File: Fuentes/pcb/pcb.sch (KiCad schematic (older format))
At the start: 16 parts, among them P1 entrada1, P2 entrada 2, P3 +50V, P4 -50V

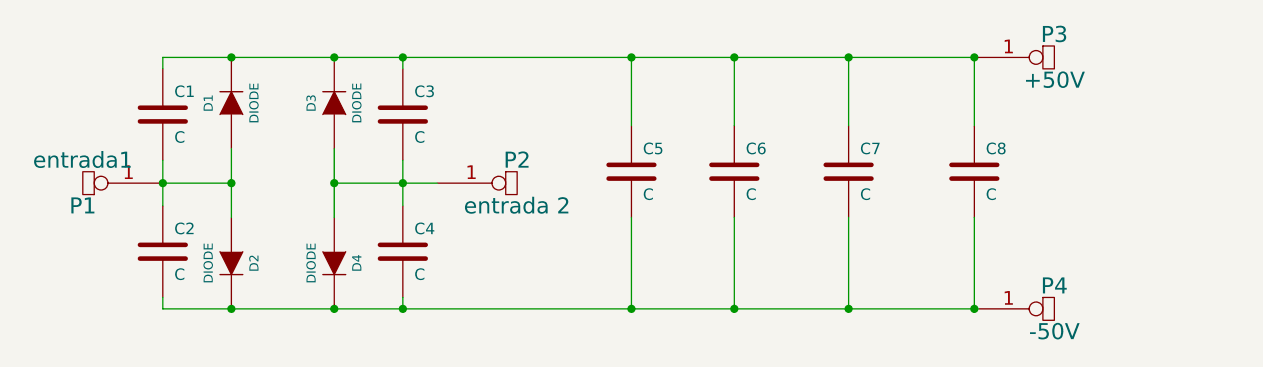
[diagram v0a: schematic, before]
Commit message: subo pcb de la fuente lineal 3
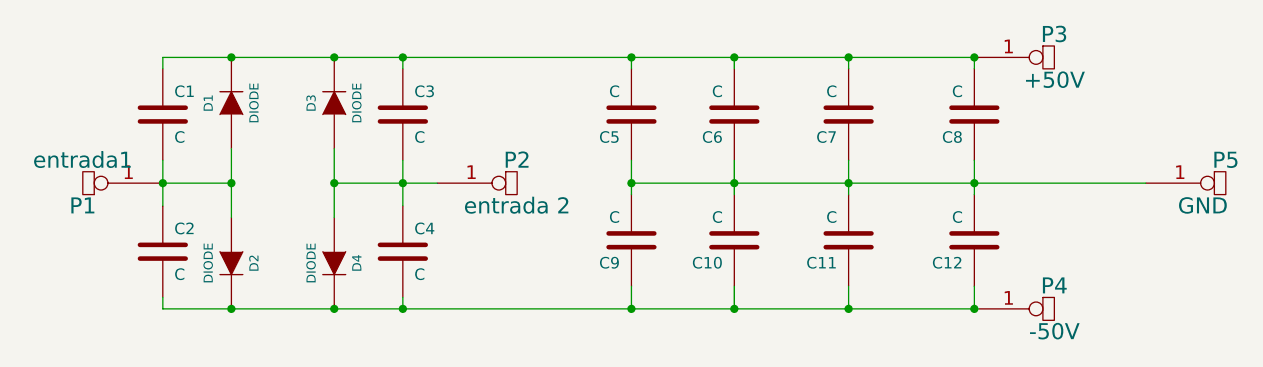
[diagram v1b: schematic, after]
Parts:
- added C10, C11, C12, C9: C, symbol C
- added P5: GND, symbol CONNECTOR
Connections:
- net at C1.1, C3.1, D1.2 (K)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: now also C5.2, C6.2, C7.2, C8.2; no longer C5.1, C6.1, C7.1, C8.1
- net at C2.2, C4.2, D2.2 (K)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: now also C10.1, C11.1, C12.1, C9.1; no longer C5.2, C6.2, C7.2, C8.2
- new net: C10.2, C11.2, C12.2, C5.1, C6.1, C7.1, C8.1, C9.2, P5.1 (W)
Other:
- moved on the sheet: C5, C6, C7, C8
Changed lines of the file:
@@
-EESchema Schematic File Version 2  date jue 31 may 2012 13:24:02 ART
+EESchema Schematic File Version 2  date jue 31 may 2012 14:37:13 ART
 LIBS:power
 LIBS:device
@@
 Comment4 ""
 $EndDescr
+Wire Wire Line
+	3200 1200 3200 1250
+Wire Wire Line
+	4700 1250 4700 1200
+Wire Wire Line
+	3200 2200 3200 2300
+Wire Wire Line
+	4150 2300 4150 2200
+Wire Wire Line
+	3650 1650 3650 1800
+Wire Wire Line
+	4700 1800 4700 1650
+Wire Wire Line
+	3200 1800 3200 1650
+Connection ~ 4150 1200
+Connection ~ 3650 2300
+Connection ~ 3200 1200
+Wire Wire Line
+	4700 1200 1150 1200
+Connection ~ 2200 2300
+Wire Wire Line
+	2200 2300 2200 2250
+Connection ~ 1450 2300
+Wire Wire Line
+	1150 2250 1150 2300
+Wire Wire Line
+	2200 1650 2200 1850
+Wire Wire Line
+	1150 1650 1150 1850
+Connection ~ 1900 1750
+Wire Wire Line
+	1900 1750 2350 1750
+Wire Wire Line
+	1450 1600 1450 1900
+Wire Wire Line
+	1900 1900 1900 1600
+Wire Wire Line
+	1450 1750 1150 1750
+Connection ~ 1450 1750
+Wire Wire Line
+	1150 1200 1150 1250
+Connection ~ 1450 1200
+Wire Wire Line
+	2200 1250 2200 1200
+Connection ~ 2200 1200
+Connection ~ 2200 1750
+Connection ~ 1150 1750
+Connection ~ 1900 2300
+Connection ~ 1900 1200
+Connection ~ 3200 2300
+Wire Wire Line
+	1150 2300 4700 2300
+Connection ~ 4150 2300
+Connection ~ 3650 1200
+Connection ~ 4700 2300
 Connection ~ 4700 1200
-Connection ~ 4700 2300
+Wire Wire Line
+	3200 1750 5450 1750
+Connection ~ 3200 1750
+Wire Wire Line
+	4150 1800 4150 1650
+Wire Wire Line
+	3650 2200 3650 2300
+Wire Wire Line
+	4700 2300 4700 2200
+Connection ~ 4700 1750
+Connection ~ 4150 1750
+Connection ~ 3650 1750
+Wire Wire Line
+	4150 1250 4150 1200
+Wire Wire Line
+	3650 1250 3650 1200
+$Comp
+L CONNECTOR P5
+U 1 1 4FC7AB52
+P 5450 1750
+F 0 "P5" H 5800 1850 70  0000 C CNN
+F 1 "GND" H 5700 1650 70  0000 C CNN
+	1    5450 1750
+	1    0    0    -1
+$EndComp
+$Comp
+L C C9
+U 1 1 4FC7AB35
+P 3200 2000
+F 0 "C9" H 3250 2100 50  0000 L CNN
+F 1 "C" H 3250 1900 50  0000 L CNN
+	1    3200 2000
+	-1   0    0    1
+$EndComp
+$Comp
+L C C10
+U 1 1 4FC7AB34
+P 3650 2000
+F 0 "C10" H 3700 2100 50  0000 L CNN
+F 1 "C" H 3700 1900 50  0000 L CNN
+	1    3650 2000
+	-1   0    0    1
+$EndComp
+$Comp
+L C C11
+U 1 1 4FC7AB33
+P 4150 2000
+F 0 "C11" H 4200 2100 50  0000 L CNN
+F 1 "C" H 4200 1900 50  0000 L CNN
+	1    4150 2000
+	-1   0    0    1
+$EndComp
+$Comp
+L C C12
+U 1 1 4FC7AB32
+P 4700 2000
+F 0 "C12" H 4750 2100 50  0000 L CNN
+F 1 "C" H 4750 1900 50  0000 L CNN
+	1    4700 2000
+	-1   0    0    1
+$EndComp
 $Comp
 L CONNECTOR P3
@@
 	1    0    0    -1
 $EndComp
-Connection ~ 3650 1200
-Wire Wire Line
-	3650 1500 3650 1200
-Connection ~ 4150 2300
-Wire Wire Line
-	4700 2300 1150 2300
-Wire Wire Line
-	4700 2300 4700 1900
-Connection ~ 3200 2300
-Wire Wire Line
-	3650 2300 3650 1900
-Connection ~ 1900 1200
-Wire Wire Line
-	3200 1200 3200 1500
-Connection ~ 1900 2300
-Connection ~ 1150 1750
-Connection ~ 2200 1750
-Connection ~ 2200 1200
-Wire Wire Line
-	2200 1250 2200 1200
-Connection ~ 1450 1200
-Wire Wire Line
-	1150 1250 1150 1200
-Connection ~ 1450 1750
-Wire Wire Line
-	1450 1750 1150 1750
-Wire Wire Line
-	1900 1900 1900 1600
-Wire Wire Line
-	1450 1600 1450 1900
-Wire Wire Line
-	1900 1750 2350 1750
-Connection ~ 1900 1750
-Wire Wire Line
-	1150 1650 1150 1850
-Wire Wire Line
-	2200 1650 2200 1850
-Wire Wire Line
-	1150 2300 1150 2250
-Connection ~ 1450 2300
-Wire Wire Line
-	2200 2300 2200 2250
-Connection ~ 2200 2300
-Wire Wire Line
-	3200 2300 3200 1900
-Wire Wire Line
-	4700 1500 4700 1200
-Wire Wire Line
-	4700 1200 1150 1200
-Connection ~ 3200 1200
-Wire Wire Line
-	4150 2300 4150 1900
-Connection ~ 3650 2300
-Wire Wire Line
-	4150 1500 4150 1200
-Connection ~ 4150 1200
 $Comp
 L C C8
 U 1 1 4FC785F8
-P 4700 1700
-F 0 "C8" H 4750 1800 50  0000 L CNN
-F 1 "C" H 4750 1600 50  0000 L CNN
-	1    4700 1700
-	1    0    0    -1
+P 4700 1450
+F 0 "C8" H 4750 1550 50  0000 L CNN
+F 1 "C" H 4750 1350 50  0000 L CNN
+	1    4700 1450
+	-1   0    0    1
 $EndComp
 $Comp
 L C C7
 U 1 1 4FC785F7
-P 4150 1700
-F 0 "C7" H 4200 1800 50  0000 L CNN
-F 1 "C" H 4200 1600 50  0000 L CNN
-	1    4150 1700
-	1    0    0    -1
+P 4150 1450
+F 0 "C7" H 4200 1550 50  0000 L CNN
+F 1 "C" H 4200 1350 50  0000 L CNN
+	1    4150 1450
+	-1   0    0    1
 $EndComp
 $Comp
 L C C6
 U 1 1 4FC78069
-P 3650 1700
-F 0 "C6" H 3700 1800 50  0000 L CNN
-F 1 "C" H 3700 1600 50  0000 L CNN
-	1    3650 1700
-	1    0    0    -1
+P 3650 1450
+F 0 "C6" H 3700 1550 50  0000 L CNN
+F 1 "C" H 3700 1350 50  0000 L CNN
+	1    3650 1450
+	-1   0    0    1
 $EndComp
 $Comp
 L C C5
 U 1 1 4FC6E52B
-P 3200 1700
-F 0 "C5" H 3250 1800 50  0000 L CNN
-F 1 "C" H 3250 1600 50  0000 L CNN
-	1    3200 1700
-	1    0    0    -1
-$EndComp
-$Comp
+P 3200 1450
+F 0 "C5" H 3250 1550 50  0000 L CNN
+F 1 "C" H 3250 1350 50  0000 L CNN
+	1    3200 1450
+	-1   0    0    1
+$EndComp
+$Comp
